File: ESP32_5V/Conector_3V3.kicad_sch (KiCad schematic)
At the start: 6 parts, among them J12 Conn_01x11, J13 Conn_01x11, J14 Conn_01x11, J7 Conn_01x11, J8 Conn_01x11, J9 Conn_01x11

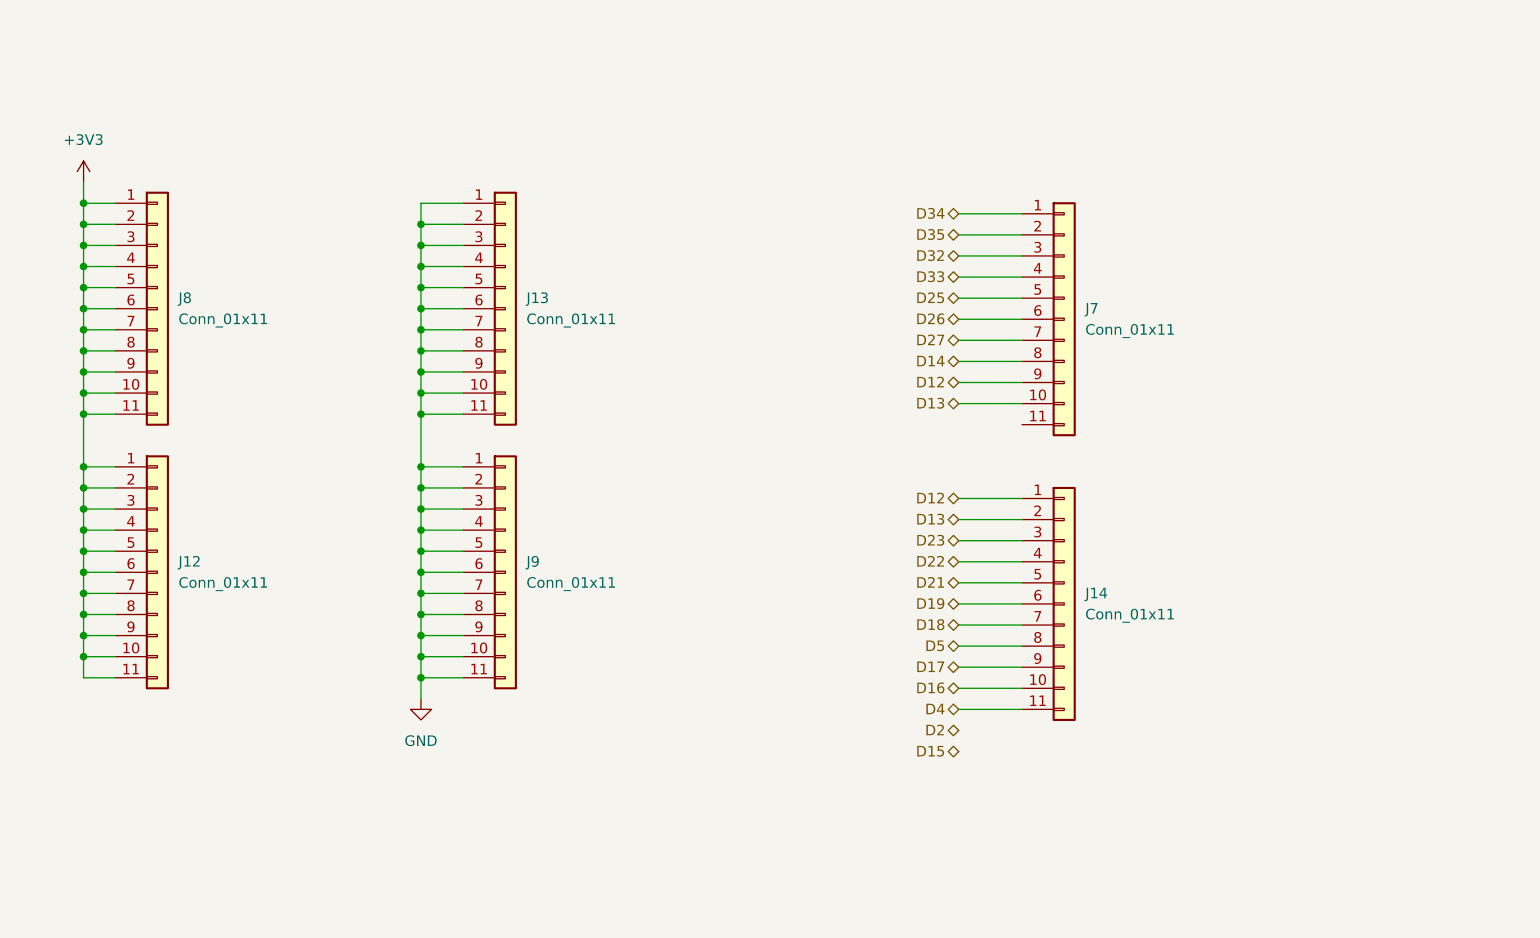
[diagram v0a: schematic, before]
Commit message: update
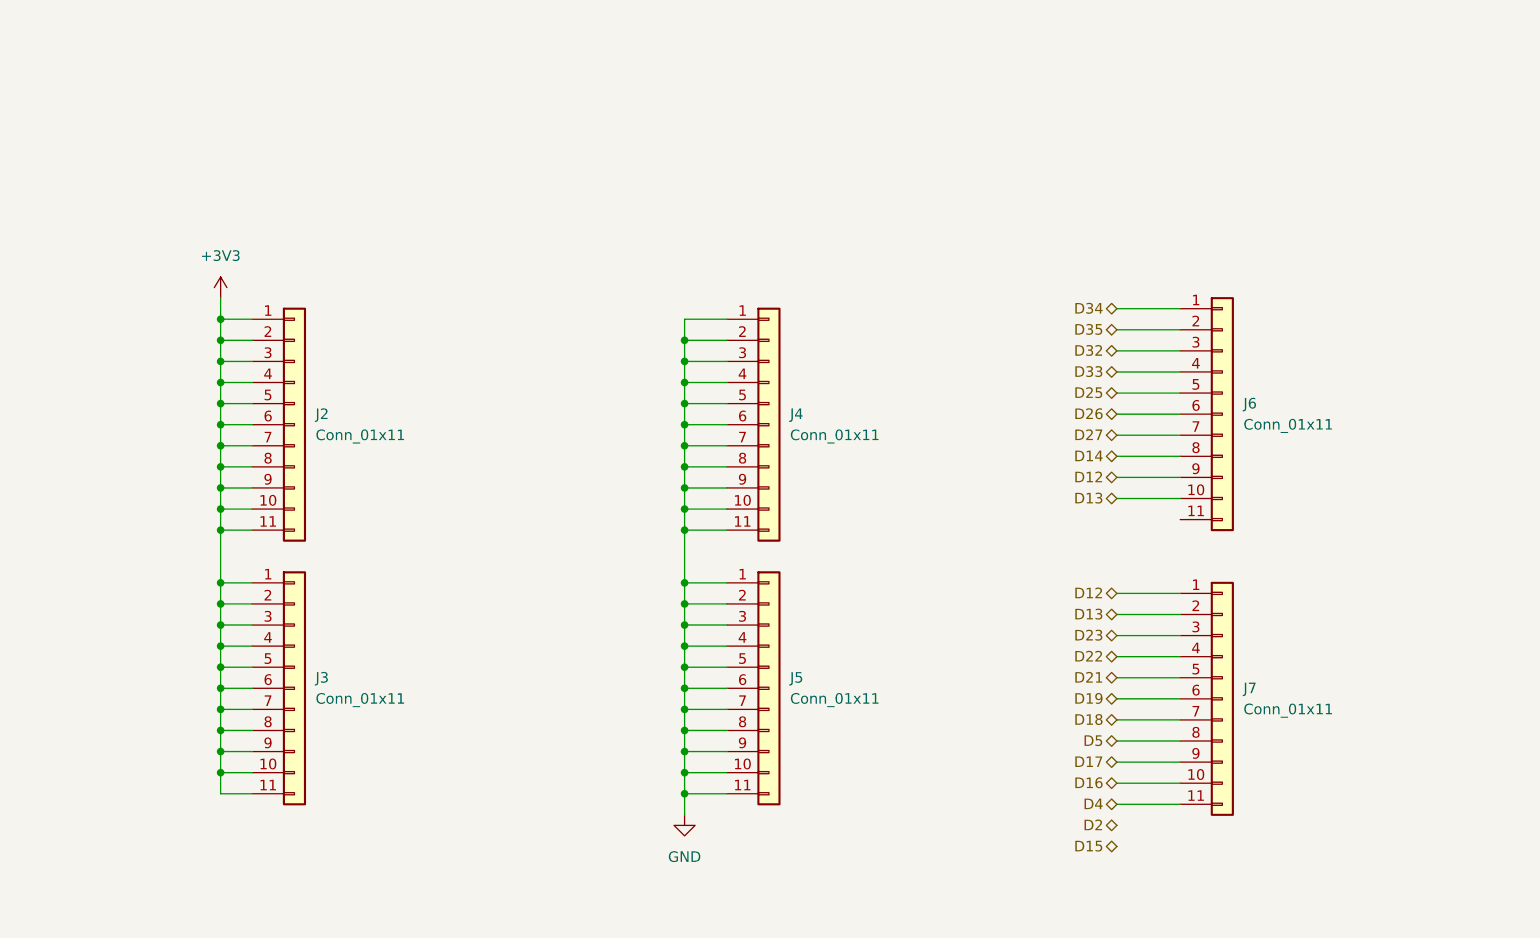
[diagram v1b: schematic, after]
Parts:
- renumbered J8 to J2, J12 to J3, J13 to J4, J9 to J5, J7 to J6, J14 to J7
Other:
- moved on the sheet: J2, J3, J4, J5, J6, J7

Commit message: update
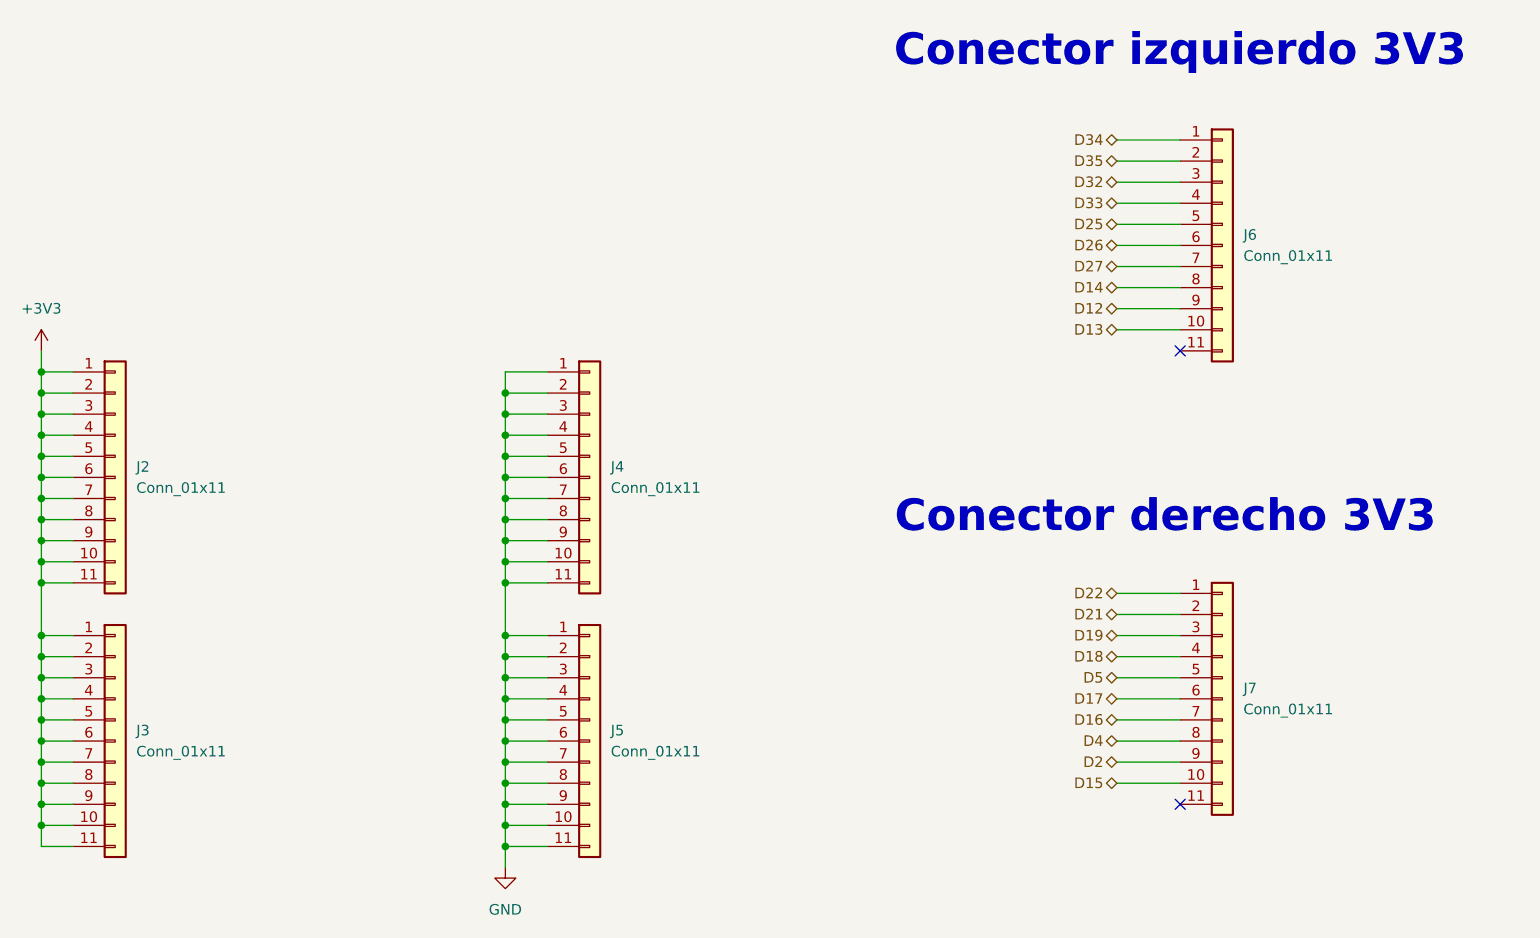
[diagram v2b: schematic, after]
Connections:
- net D23 is gone; now on net D19: J7.3 (Pin_3)
- net D12: no longer J7.1 (Pin_1)
- net D13: no longer J7.2 (Pin_2)
- net D15: now also J7.10 (Pin_10)
- net D16: now also J7.7 (Pin_7); no longer J7.10 (Pin_10)
- net D17: now also J7.6 (Pin_6); no longer J7.9 (Pin_9)
- net D18: now also J7.4 (Pin_4); no longer J7.7 (Pin_7)
- net D19: no longer J7.6 (Pin_6)
- net D2: now also J7.9 (Pin_9)
- net D21: now also J7.2 (Pin_2); no longer J7.5 (Pin_5)
- net D22: now also J7.1 (Pin_1); no longer J7.4 (Pin_4)
- net D4: now also J7.8 (Pin_8); no longer J7.11 (Pin_11)
- net D5: now also J7.5 (Pin_5); no longer J7.8 (Pin_8)
- no-connect marks 0 -> 2
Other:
- note added: "Conector derecho 3V3"
- note added: "Conector izquierdo 3V3"
- moved on the sheet: J2, J3, J4, J5, J6
